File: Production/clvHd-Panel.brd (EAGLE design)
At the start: 113 x 82.7 mm, 334 parts, among them IC1 LMV324M, IC2 LMV324M, IC3 LMV324M, IC4 LMV324M, IC5 LMV324M, IC6 LMV324M, IC7 LMV324M, IC8 LMV324M, X1 009176002, X10 009176002, X11 009176002, X12 SSW-101-02-G-S, X13 SSW-101-02-G-S, X14 SSW-101-02-G-S, X15 009176002, X16 009176002, X17 009176002, X18 009176002, X19 SSW-101-02-G-S, X2 009176002, X20 SSW-101-02-G-S, X21 SSW-101-02-G-S, X22 009176002, X23 009176002, X24 009176002, X25 009176002, X26 SSW-101-02-G-S, X27 SSW-101-02-G-S, X28 SSW-101-02-G-S, X29 009176002, X3 SSW-101-02-G-S, X30 009176002, X31 009176002, X32 009176002, X33 SSW-101-02-G-S, X34 SSW-101-02-G-S, X35 SSW-101-02-G-S, X36 009176002, X37 009176002, X38 009176002, X39 009176002, X4 009176002, X40 SSW-101-02-G-S, X41 SSW-101-02-G-S, X42 SSW-101-02-G-S, X43 009176002, X44 009176002, X45 009176002, X46 009176002, X47 SSW-101-02-G-S, X48 SSW-101-02-G-S, X49 SSW-101-02-G-S, X5 SSW-101-02-G-S, X50 009176002, X51 009176002, X52 009176002, X53 009176002, X54 SSW-101-02-G-S, X55 SSW-101-02-G-S, X56 SSW-101-02-G-S, X6 009176002, X7 SSW-101-02-G-S, X8 009176002, X9 009176002

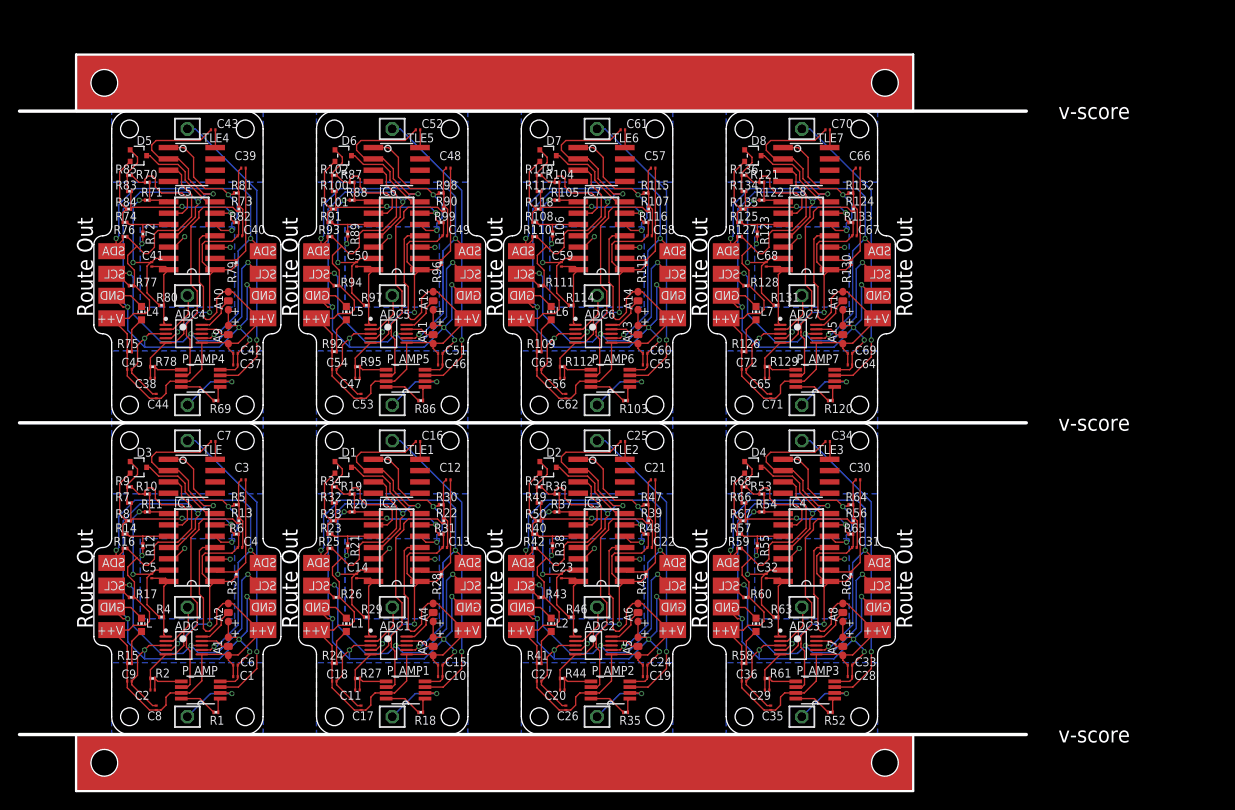
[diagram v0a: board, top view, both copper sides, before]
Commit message: panelized
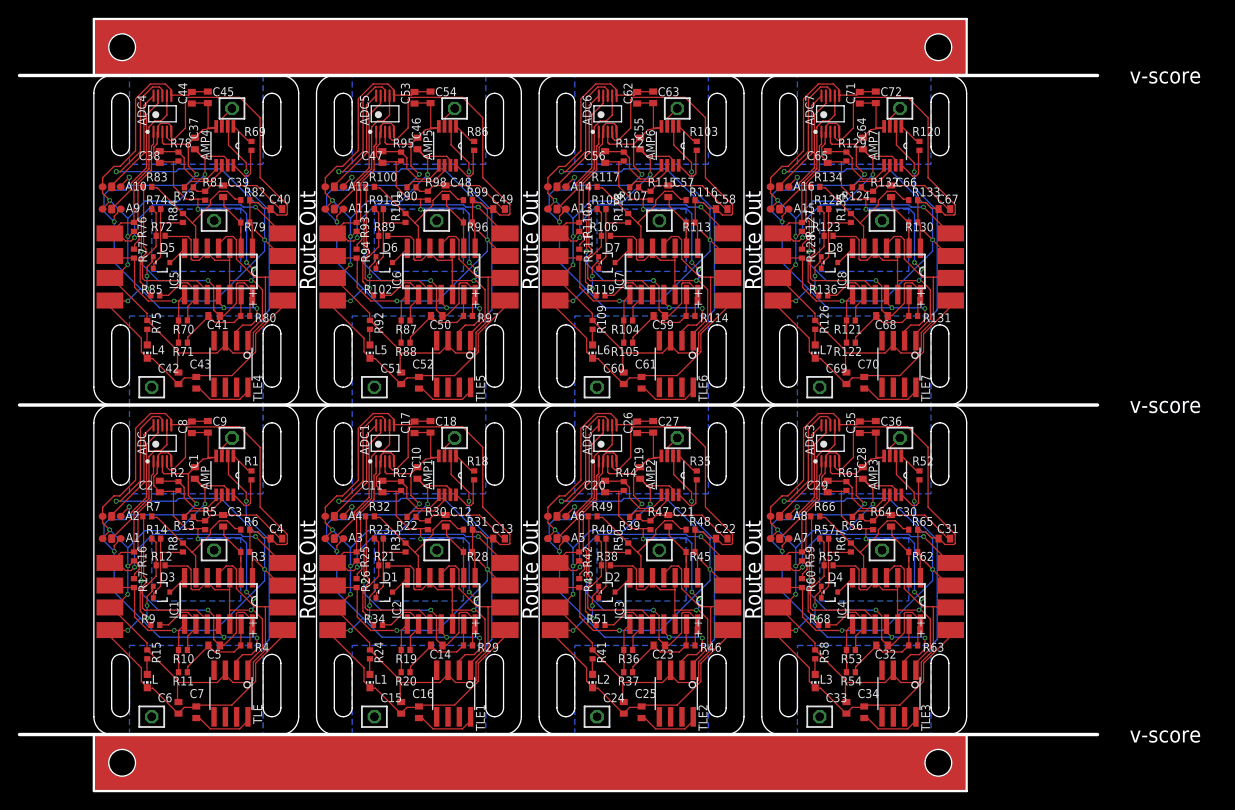
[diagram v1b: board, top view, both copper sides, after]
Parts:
- removed P_AMP, P_AMP1, P_AMP2, P_AMP3, P_AMP4, P_AMP5, P_AMP6, P_AMP7: INA326EA/250, INA326EA_250:SOP65P490X110-8N
- added AMP, AMP1, AMP2, AMP3, AMP4, AMP5, AMP6, AMP7: INA326EA/250, INA326EA_250:SOP65P490X110-8N
- C1, C10, C11, C12, C13, C14, C15, C16, C17, C18, C19, C2, C20, C21, C22, C23, C24, C25, C26, C27, C28, C29, C3, C30, C31, C32, C33, C34, C35, C36, C37, C38, C39, C4, C40, C41, C42, C43, C44, C45, C46, C47, C48, C49, C5, C50, C51, C52, C53, C54, C55, C56, C57, C58, C59, C6, C60, C61, C62, C63, C64, C65, C66, C67, C68, C69, C7, C70, C71, C72, C8, C9: device rcl:C0201 -> rcl:C0402
- R1, R10, R100, R101, R102, R103, R104, R105, R106, R107, R108, R109, R11, R110, R111, R112, R113, R114, R115, R116, R117, R118, R119, R12, R120, R121, R122, R123, R124, R125, R126, R127, R128, R129, R13, R130, R131, R132, R133, R134, R135, R136, R14, R15, R16, R17, R18, R19, R2, R20, R21, R22, R23, R24, R25, R26, R27, R28, R29, R3, R30, R31, R32, R33, R34, R35, R36, R37, R38, R39, R4, R40, R41, R42, R43, R44, R45, R46, R47, R48, R49, R5, R50, R51, R52, R53, R54, R55, R56, R57, R58, R59, R6, R60, R61, R62, R63, R64, R65, R66, R67, R68, R69, R7, R70, R71, R72, R73, R74, R75, R76, R77, R78, R79, R8, R80, R81, R82, R83, R84, R85, R86, R87, R88, R89, R9, R90, R91, R92, R93, R94, R95, R96, R97, R98, R99: device rcl:R0201 -> rcl:R0402
- moved C71 35.0 mm to (86.0, 71.5), turned to 90 degrees
- moved C62 34.4 mm to (61.0, 71.5), turned to 90 degrees
- moved C53 34.0 mm to (36.0, 71.5), turned to 90 degrees
- moved C72 33.9 mm to (87.8, 71.6), turned to 90 degrees
- moved C44 33.7 mm to (11.0, 71.5), turned to 90 degrees
- moved C63 33.1 mm to (62.8, 71.6), turned to 90 degrees
- moved C35 33.0 mm to (86.0, 34.5), turned to 90 degrees
- moved C26 32.5 mm to (61.0, 34.5), turned to 90 degrees
- moved C54 32.4 mm to (37.8, 71.6), turned to 90 degrees
- moved C36 32.2 mm to (87.8, 34.5), turned to 90 degrees
- moved C17 32.1 mm to (36.0, 34.5), turned to 90 degrees
- moved C45 31.8 mm to (12.8, 71.6), turned to 90 degrees
- moved C8 31.8 mm to (11.0, 34.5), turned to 90 degrees
- moved C27 31.3 mm to (62.8, 34.5), turned to 90 degrees
- moved C34 30.7 mm to (86.5, 2.50), turned to 90 degrees
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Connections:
- net INM: now also AMP.2; no longer P_AMP.2
- net INM1: now also AMP1.2; no longer P_AMP1.2
- net INM2: now also AMP2.2; no longer P_AMP2.2
- net INM3: now also AMP3.2; no longer P_AMP3.2
- net INM4: now also AMP4.2; no longer P_AMP4.2
- net INM5: now also AMP5.2; no longer P_AMP5.2
- net INM6: now also AMP6.2; no longer P_AMP6.2
- net INM7: now also AMP7.2; no longer P_AMP7.2
- net INP: now also AMP.3; no longer P_AMP.3
- net INP1: now also AMP1.3; no longer P_AMP1.3
- net INP2: now also AMP2.3; no longer P_AMP2.3
- net INP3: now also AMP3.3; no longer P_AMP3.3
- net INP4: now also AMP4.3; no longer P_AMP4.3
- net INP5: now also AMP5.3; no longer P_AMP5.3
- net INP6: now also AMP6.3; no longer P_AMP6.3
- net INP7: now also AMP7.3; no longer P_AMP7.3
- net N$1: now also AMP.1; no longer P_AMP.1
- net N$100: now also AMP4.6; no longer P_AMP4.6
- net N$101: now also AMP4.1; no longer P_AMP4.1
- net N$102: now also AMP4.8; no longer P_AMP4.8
- net N$116: now also AMP5.5; no longer P_AMP5.5
- net N$122: now also AMP5.6; no longer P_AMP5.6
- net N$123: now also AMP5.1; no longer P_AMP5.1
- net N$124: now also AMP5.8; no longer P_AMP5.8
- net N$138: now also AMP6.5; no longer P_AMP6.5
- net N$144: now also AMP6.6; no longer P_AMP6.6
- net N$145: now also AMP6.1; no longer P_AMP6.1
- net N$146: now also AMP6.8; no longer P_AMP6.8
- net N$160: now also AMP7.5; no longer P_AMP7.5
- net N$166: now also AMP7.6; no longer P_AMP7.6
- net N$167: now also AMP7.1; no longer P_AMP7.1
- net N$168: now also AMP7.8; no longer P_AMP7.8
- net N$2: now also AMP.8; no longer P_AMP.8
- net N$22: now also AMP1.5; no longer P_AMP1.5
- net N$29: now also AMP1.6; no longer P_AMP1.6
- net N$30: now also AMP1.1; no longer P_AMP1.1
- net N$31: now also AMP1.8; no longer P_AMP1.8
- net N$4: now also AMP.5; no longer P_AMP.5
- net N$45: now also AMP2.5; no longer P_AMP2.5
- net N$51: now also AMP2.6; no longer P_AMP2.6
- net N$52: now also AMP2.1; no longer P_AMP2.1
- net N$53: now also AMP2.8; no longer P_AMP2.8
- net N$72: now also AMP3.5; no longer P_AMP3.5
- net N$78: now also AMP3.6; no longer P_AMP3.6
- net N$79: now also AMP3.1; no longer P_AMP3.1
- net N$80: now also AMP3.8; no longer P_AMP3.8
- net N$9: now also AMP.6; no longer P_AMP.6
- net N$94: now also AMP4.5; no longer P_AMP4.5
- net V+: now also AMP.7; no longer P_AMP.7
- net V+1: now also AMP1.7; no longer P_AMP1.7
- net V+2: now also AMP2.7; no longer P_AMP2.7
- net V+3: now also AMP3.7; no longer P_AMP3.7
- net V+4: now also AMP4.7; no longer P_AMP4.7
- net V+5: now also AMP5.7; no longer P_AMP5.7
- net V+6: now also AMP6.7; no longer P_AMP6.7
- net V+7: now also AMP7.7; no longer P_AMP7.7
- net V-: now also AMP.4; no longer P_AMP.4
- net V-1: now also AMP1.4; no longer P_AMP1.4
- net V-2: now also AMP2.4; no longer P_AMP2.4
- net V-3: now also AMP3.4; no longer P_AMP3.4
- net V-4: now also AMP4.4; no longer P_AMP4.4
- net V-5: now also AMP5.4; no longer P_AMP5.4
- net V-6: now also AMP6.4; no longer P_AMP6.4
- net V-7: now also AMP7.4; no longer P_AMP7.4
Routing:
- net INP7: track 34.3 -> 2.50 mm, vias 1 -> 0
- net INP: track 34.3 -> 2.50 mm, vias 1 -> 0
- net INP4: track 34.3 -> 2.50 mm, vias 1 -> 0
- net INP3: track 34.3 -> 2.50 mm, vias 1 -> 0
- net INP5: track 34.3 -> 2.50 mm, vias 1 -> 0
- net INP1: track 34.3 -> 2.50 mm, vias 1 -> 0
- net INP2: track 34.3 -> 2.50 mm, vias 1 -> 0
- net INP6: track 34.3 -> 2.50 mm, vias 1 -> 0
- net N$86: track 34.4 -> 65.0 mm
- net N$174: track 34.4 -> 65.0 mm
- net N$37: track 34.4 -> 65.0 mm
- net N$152: track 34.4 -> 65.0 mm
- net N$64: track 34.4 -> 65.0 mm
- net N$130: track 34.4 -> 65.0 mm
- net N$56: track 34.4 -> 65.0 mm
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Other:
- board size 113 x 82.7 mm -> 121 x 86.7 mm
- board text added: "v8"
- board text removed: "v7"
